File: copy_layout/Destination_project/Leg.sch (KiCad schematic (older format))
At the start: 10 parts, among them Q1 CSD19531KCS, Q2 CSD19531KCS, U2 IR2181, U3 LTS_15

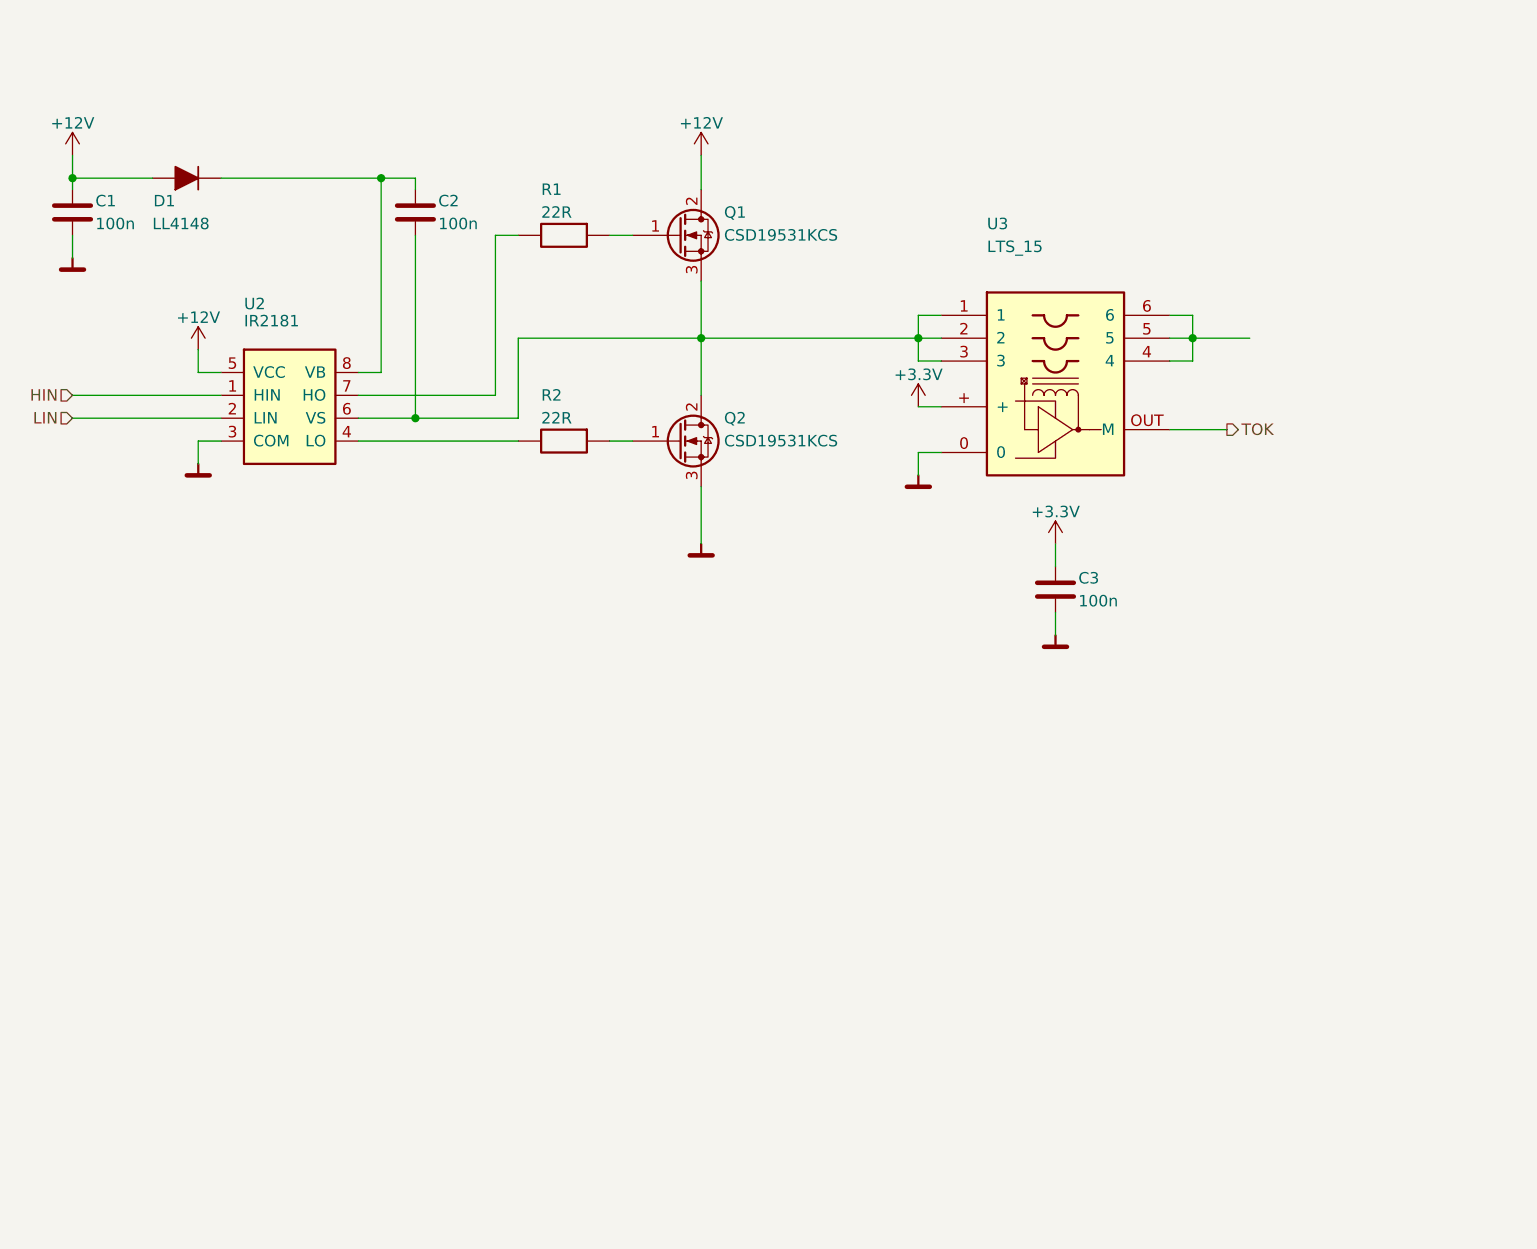
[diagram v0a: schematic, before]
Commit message: Delna verzija
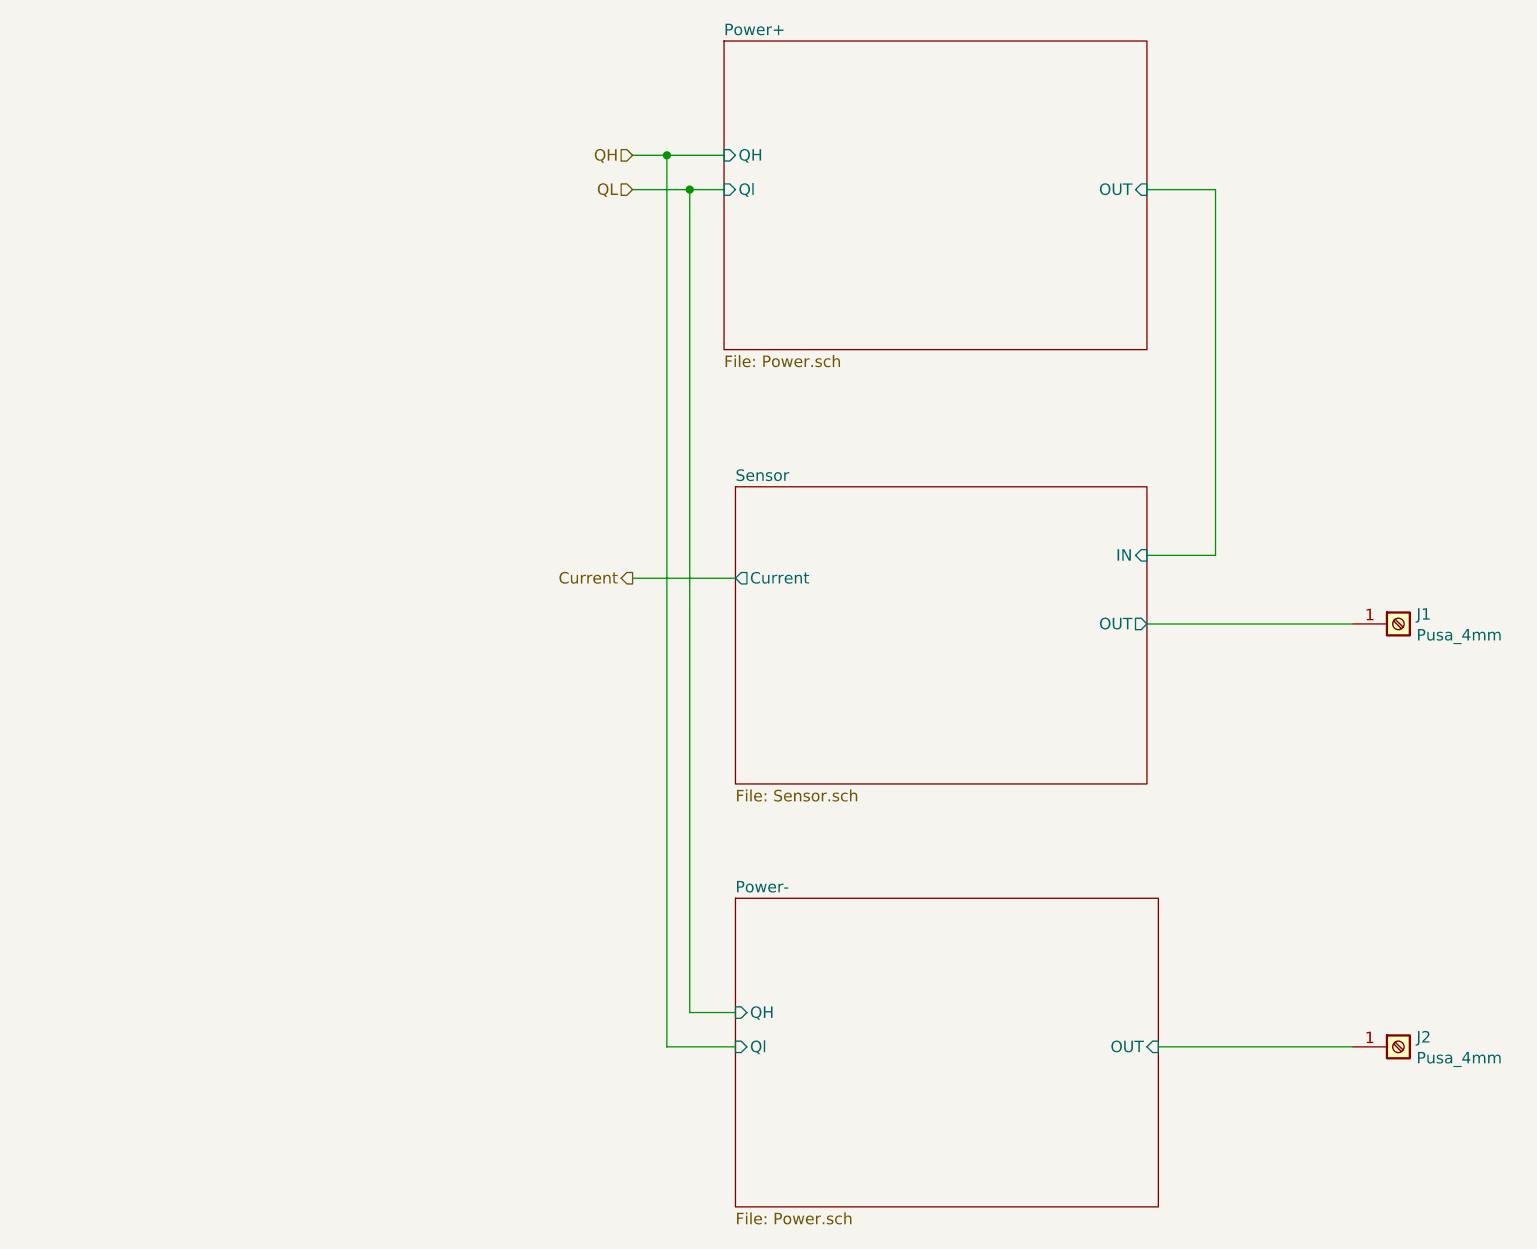
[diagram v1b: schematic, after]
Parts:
- removed C1, C2, C3: 100n, Passives:C1206M, symbol Passives:C1206
- removed D1: LL4148, Discretes:D_MiniMELF, symbol Discretes:LL4148
- removed Q1, Q2: CSD19531KCS, Discretes:TO-220, symbol Discretes:CSD19531KCS
- removed R1, R2: 22R, Passives:R1206M, symbol Passives:R1206
- removed U2: IR2181, Package_SO:SO8, symbol ICs:IR2181
- removed U3: LTS_15, Sensor_Current:LTS_15, symbol Sensor_Current:LTS_15
- added J1, J2: Pusa_4mm, Connector:Pusa_4mm, symbol Connector:Pusa_4mm
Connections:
- new net Power-/OUT: J2.1 (Pin_1)
- new net Sensor/OUT: J1.1 (Pin_1)
